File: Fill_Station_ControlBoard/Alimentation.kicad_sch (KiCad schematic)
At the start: 48 parts, among them IC2 TPS259573DSGR, J10 Screw_Terminal_2_P5.00mm, U4 TPS2116DRL, U7 OKI-78SR-5_1.5-W36-C, U8 TPS55285

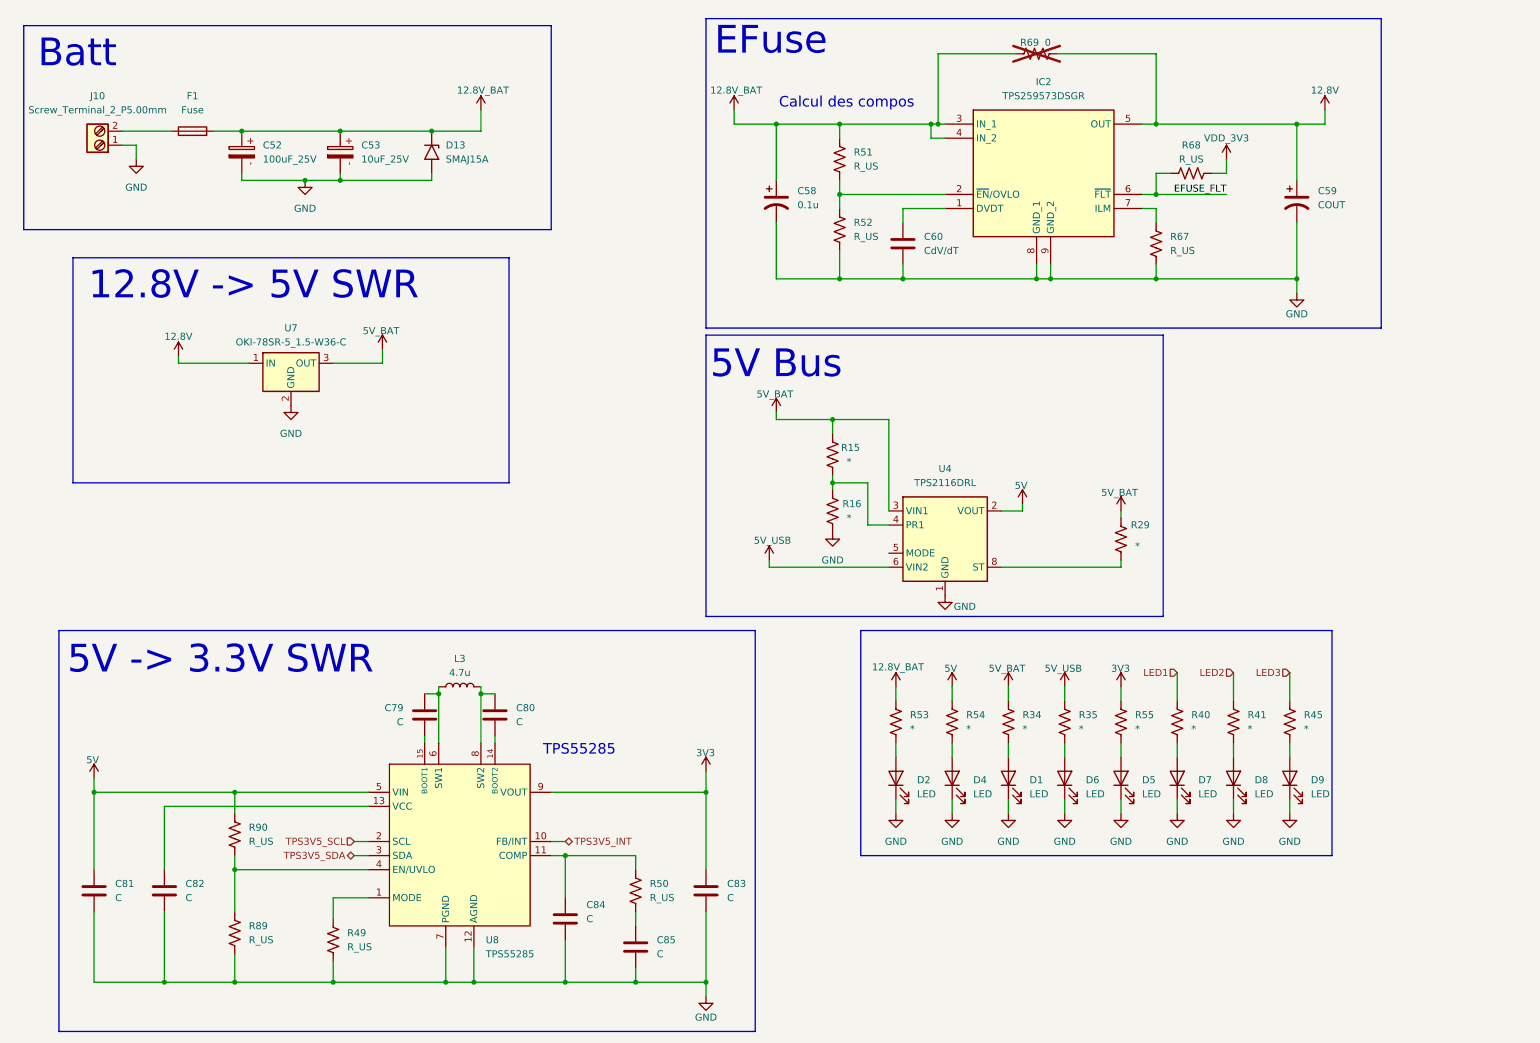
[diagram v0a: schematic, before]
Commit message: début layout
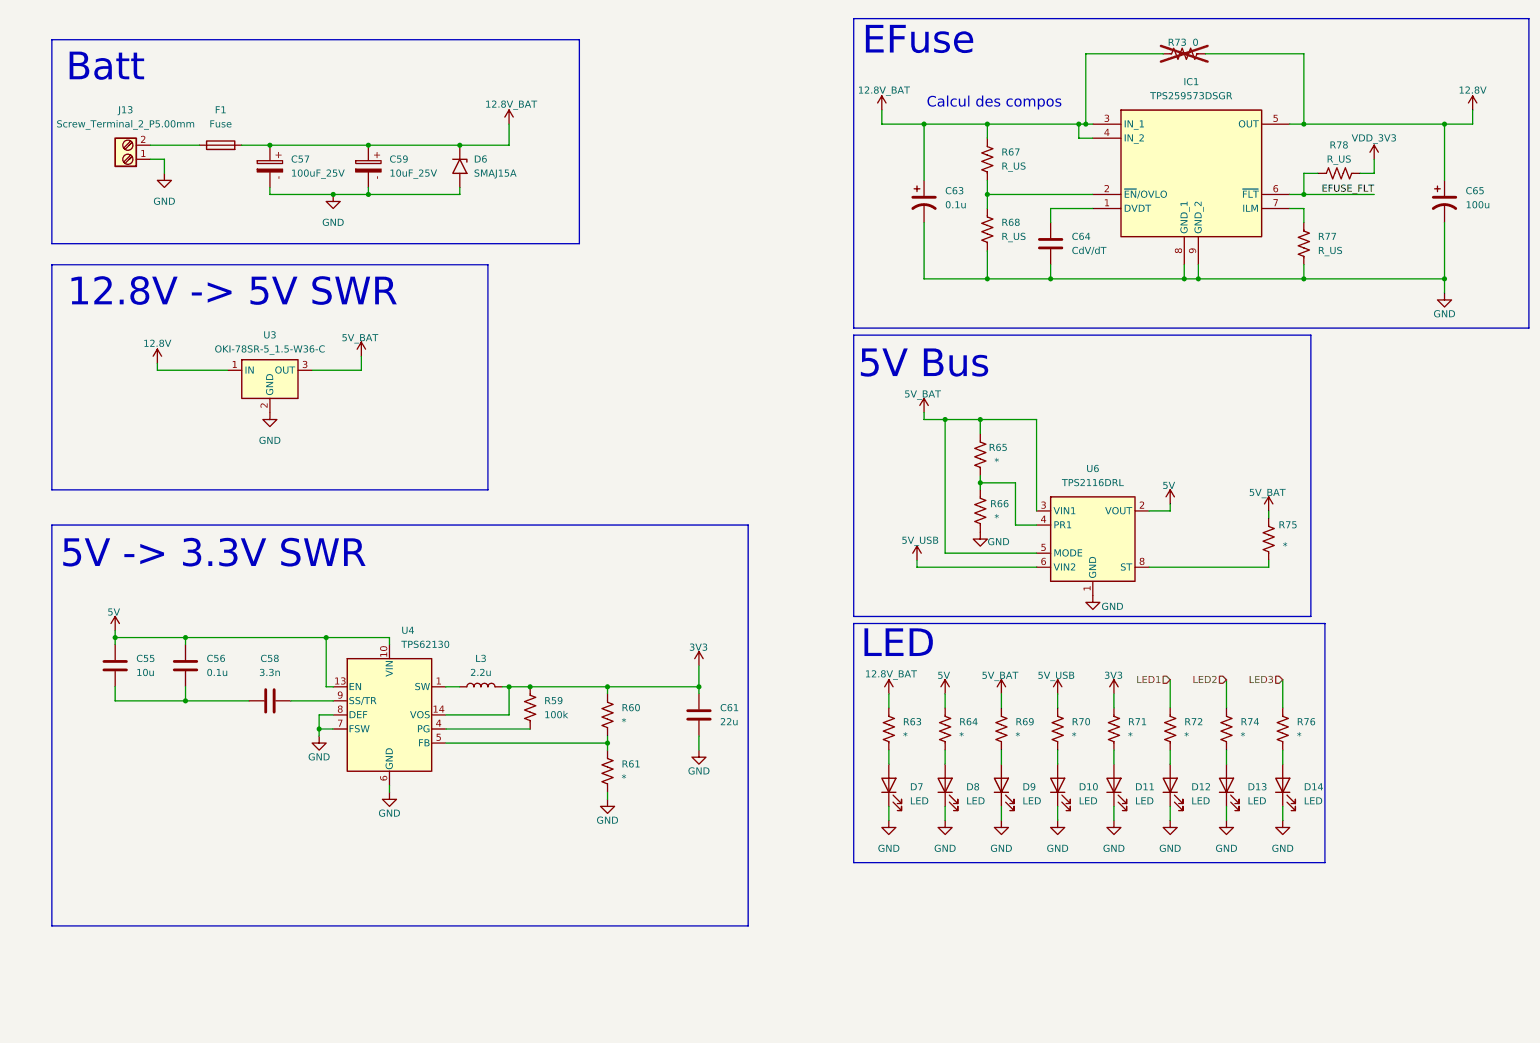
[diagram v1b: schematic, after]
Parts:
- removed C79, C80, C81, C82, C84, C85: C, Capacitor_SMD:C_0603_1608Metric, symbol Device:C
- removed R49, R50, R89, R90: R_US, Resistor_SMD:R_0603_1608Metric, symbol Device:R_US
- removed U8: TPS55285, symbol SiriusLib:TPS55285
- added C55: 10u, Capacitor_SMD:C_0603_1608Metric, symbol Device:C
- added C56: 0.1u, Capacitor_SMD:C_0603_1608Metric, symbol Device:C
- added C58: 3.3n, Capacitor_SMD:C_0603_1608Metric, symbol Device:C
- added R59: 100k, Resistor_SMD:R_0805_2012Metric, symbol Device:R_US
- added R60, R61: *, Resistor_SMD:R_0805_2012Metric, symbol Device:R_US
- added U4: TPS62130, Package_DFN_QFN:VQFN-16-1EP_3x3mm_P0.5mm_EP1.68x1.68mm_ThermalVias, symbol Regulator_Switching:TPS62130
- C61: renamed from C83; value C -> 22u
- C65: renamed from C59; value COUT -> 100u
- F1: footprint (none) -> Fuse:Fuse_0603_1608Metric
- IC1: renamed from IC2; footprint SON50P200X200X80-9N -> Package_SON:WSON-8-1EP_2x2mm_P0.5mm_EP0.9x1.6mm_ThermalVias
- L3: value 4.7u -> 2.2u
- R65: renamed from R15; footprint Resistor_SMD:R_0805_2012Metric -> Capacitor_SMD:C_0603_1608Metric
- R66: renamed from R16; footprint Resistor_SMD:R_0805_2012Metric -> Capacitor_SMD:C_0603_1608Metric
- R75: renamed from R29; footprint Resistor_SMD:R_0805_2012Metric -> Capacitor_SMD:C_0603_1608Metric
- renumbered C52 to C57, C53 to C59, C58 to C63, C60 to C64, D6 to D10, D5 to D11, D7 to D12, D8 to D13, D9 to D14, D13 to D6, D2 to D7, D4 to D8, D1 to D9, J10 to J13, R53 to R63, R54 to R64, R51 to R67, R52 to R68, R34 to R69, R35 to R70, R55 to R71, R40 to R72, R69 to R73, R41 to R74, R45 to R76, R67 to R77, R68 to R78, U7 to U3, U4 to U6
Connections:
- net 3V3: now also L3.2, R59.2, R60.2, U4.14 (VOS)
- net 5V: now also C55.1, C56.1, U4.10 (VIN), U4.11 (VIN), U4.12 (VIN), U4.13 (EN)
- net 5V_BAT: now also U6.5 (MODE)
- net GND: now also R61.1, U4.15 (GND), U4.16 (GND), U4.17 (GND), U4.6 (GND), U4.7 (FSW), U4.8 (DEF)
- net at L3.1: now also U4.1 (SW), U4.2 (SW), U4.3 (SW)
- new net: C55.2, C56.2, C58.2
- new net: R59.1, U4.4 (PG)
- new net: R60.1, R61.2, U4.5 (FB)
- new net: C58.1, U4.9 (SS/TR)
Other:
- note added: "LED"
- note removed: "TPS55285"
- moved on the sheet: C57, C59, C61, C63, C64, C65, D10, D11, D12, D13, D14, D6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
